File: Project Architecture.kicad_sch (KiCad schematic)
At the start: 40 parts, among them J1 USB4105-GF-A, Q1 PT334-6C, U1 LM393, U2 USBLC6-2SC6, U3 FT231XS-U

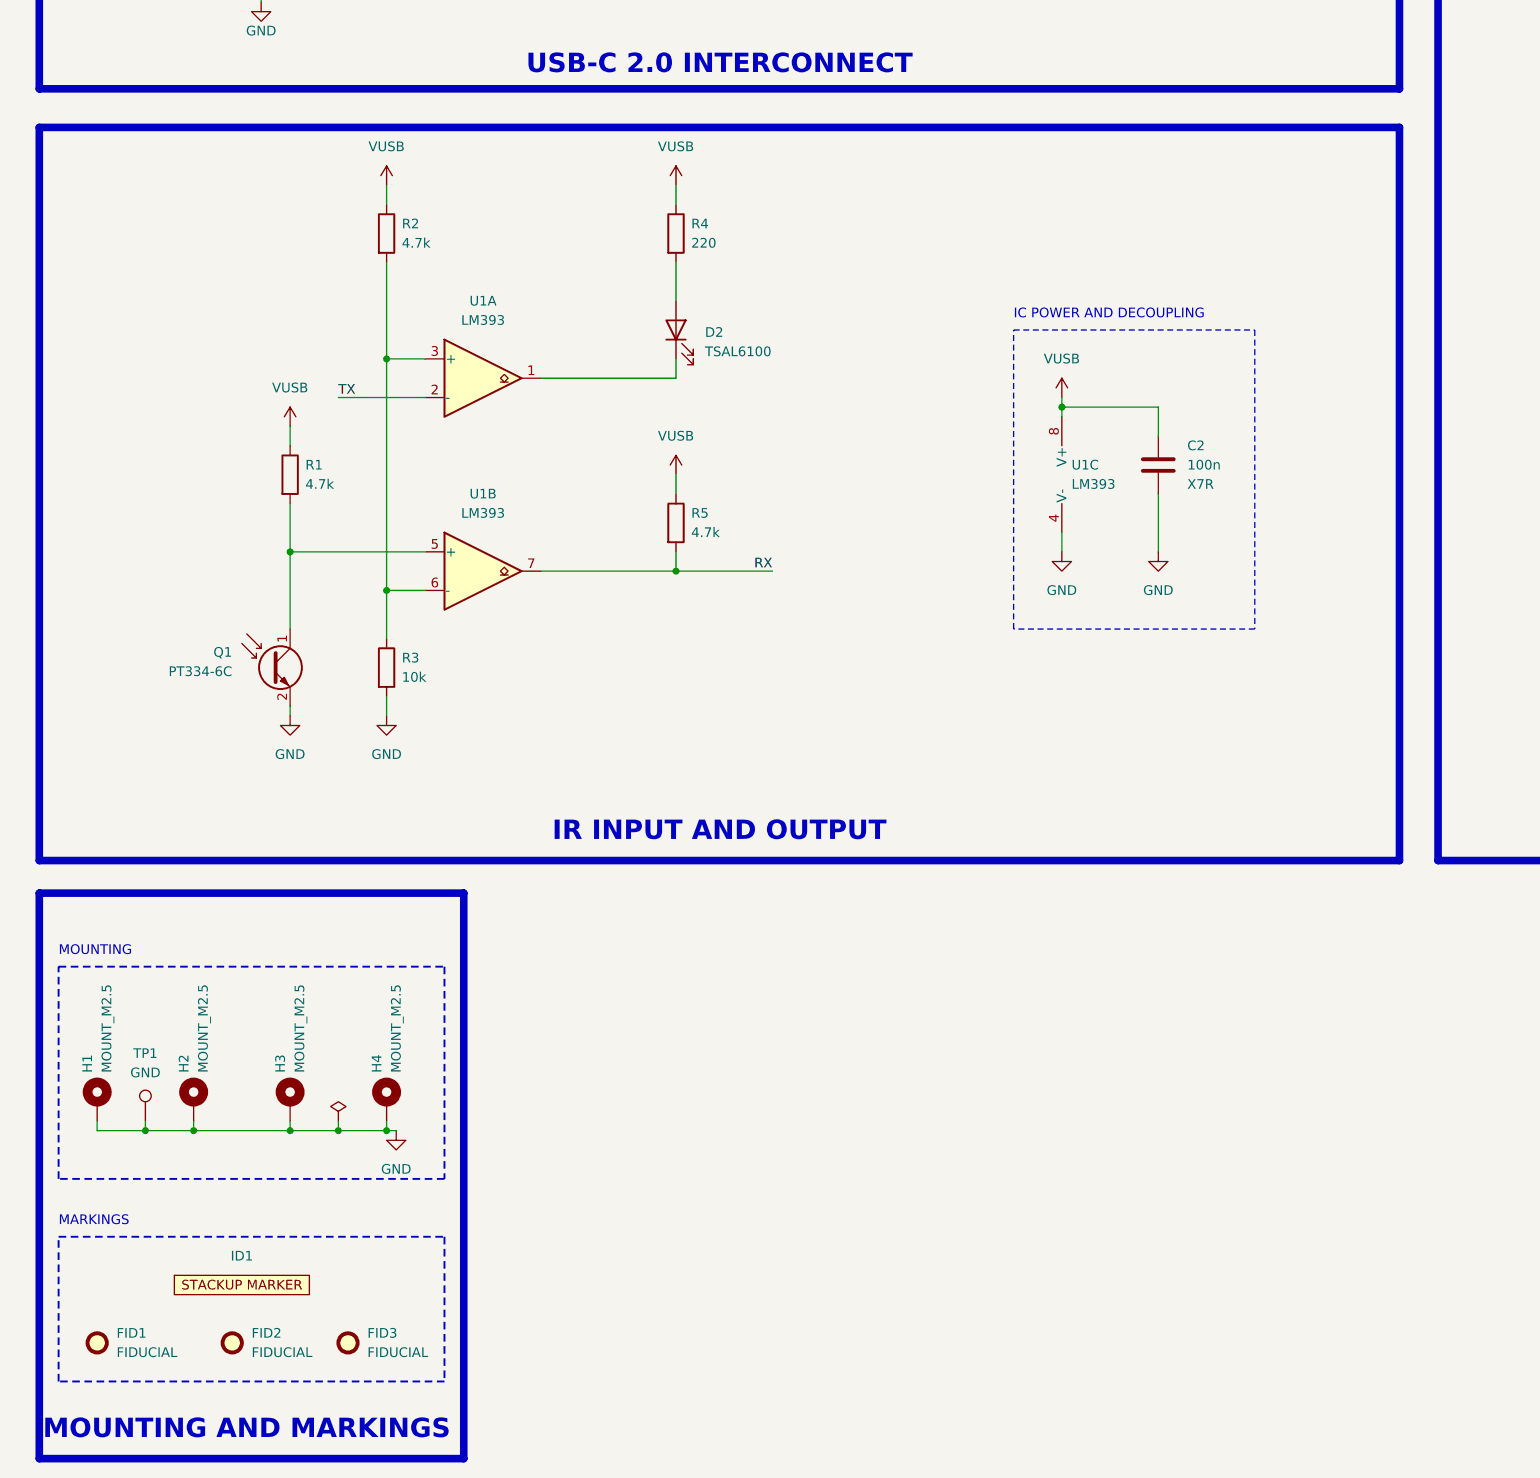
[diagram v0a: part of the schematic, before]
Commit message: feat: migrate project to Boardwright
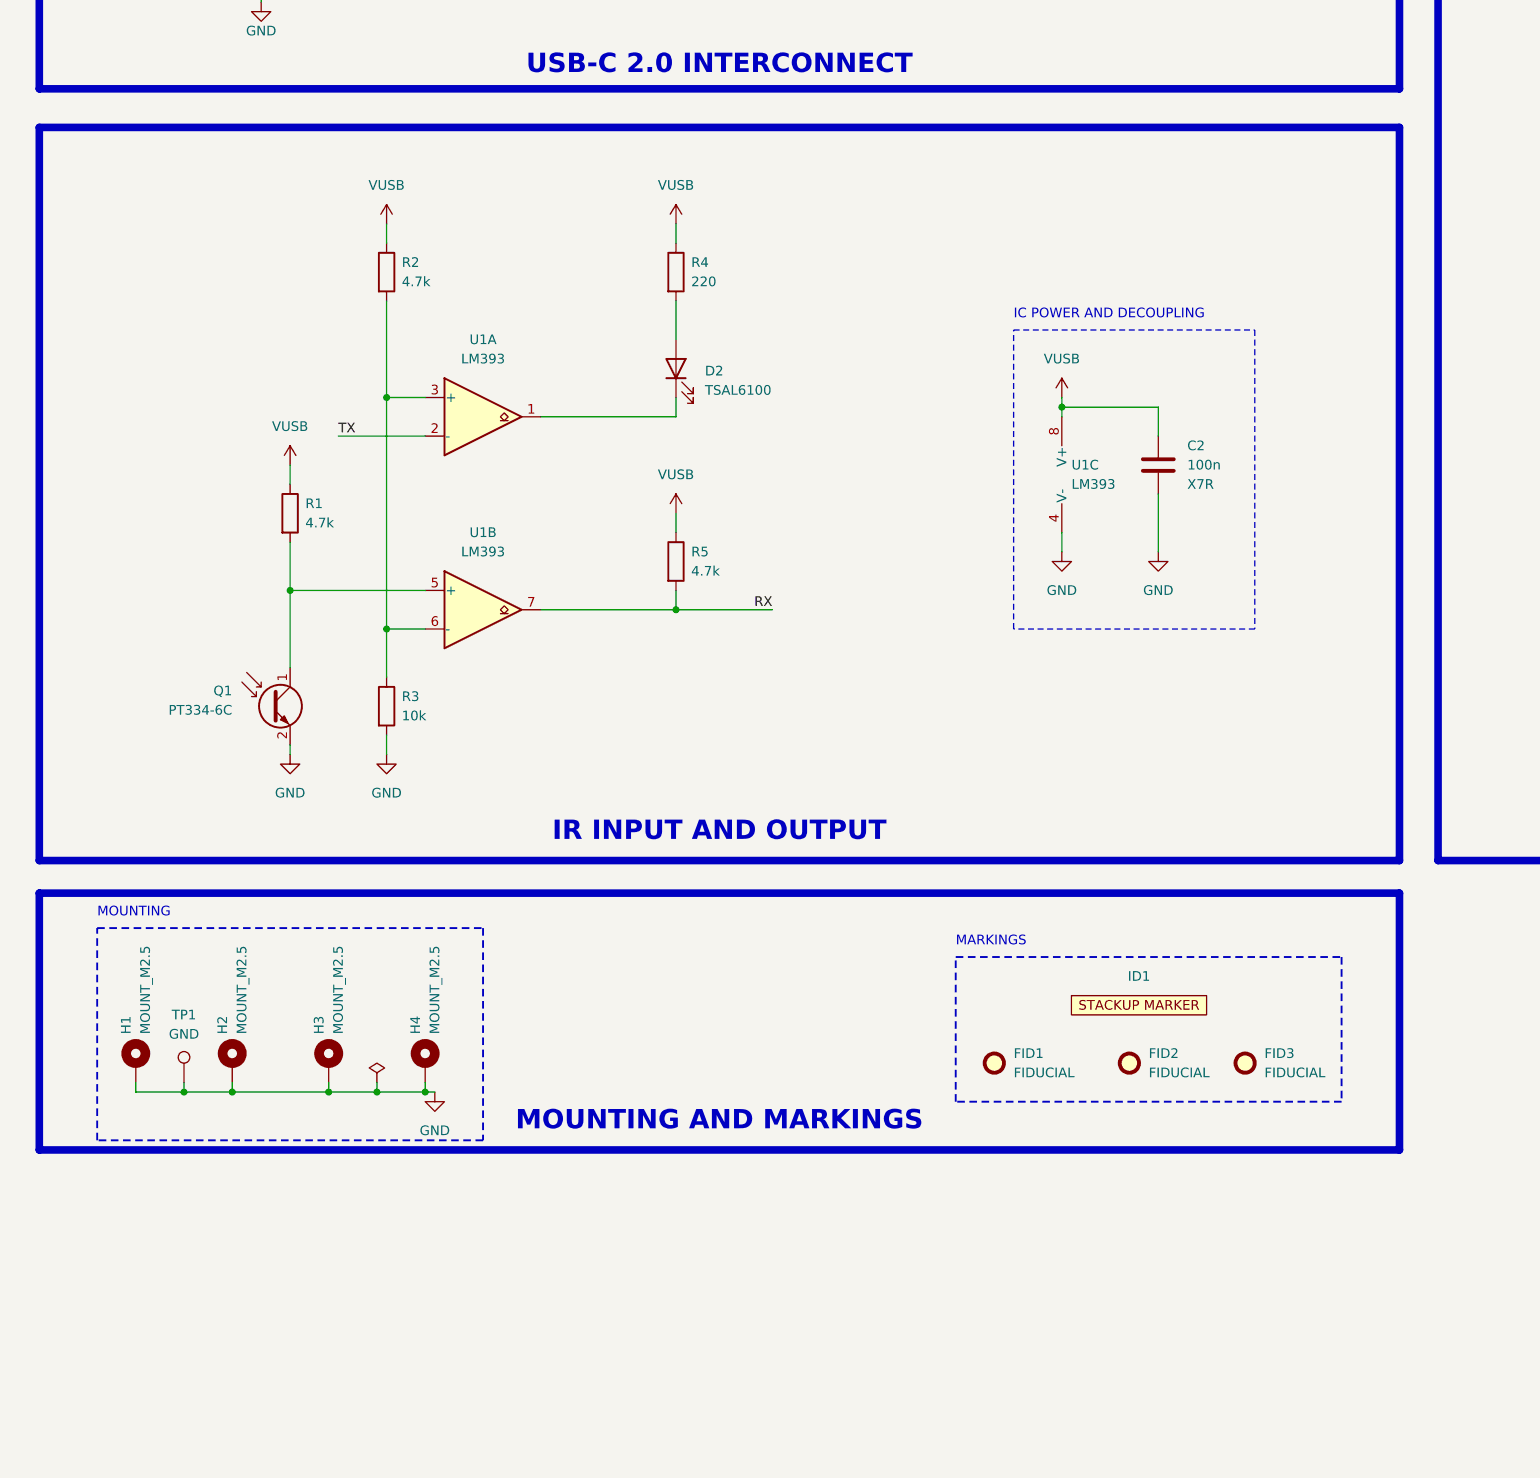
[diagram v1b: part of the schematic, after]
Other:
- moved on the sheet: D2, FID1, FID2, FID3, H1, H2, H3, H4, ID1, Q1, R1, R2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
